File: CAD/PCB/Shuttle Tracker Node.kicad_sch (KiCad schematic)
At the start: 23 parts, among them J1 Conn_01x01, J2 Conn_01x01, J3 Conn_01x01, J4 Conn_01x01, J5 Conn_01x01, J6 Conn_01x01, J7 Conn_01x01, SW1 SW_Push, SW10 SW_Push, SW11 SW_Push, SW12 SW_Push, SW13 PEC11-4215F-S24, SW2 SW_Push, SW3 SW_Push, SW4 SW_Push, SW5 SW_Push, SW6 SW_Push, SW7 SW_Push, SW8 SW_Push, SW9 SW_Push, U1 ESP32-C3-DEVKITC-02

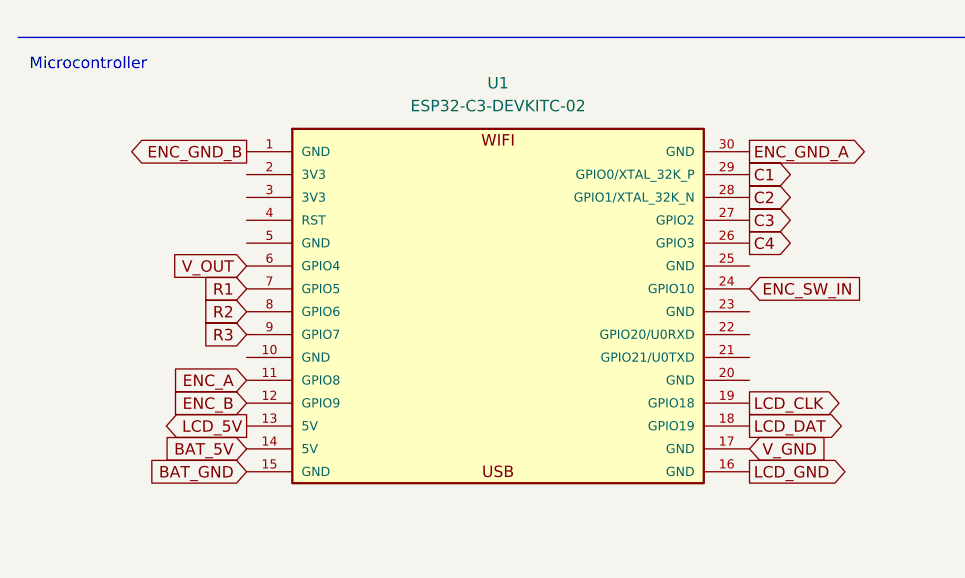
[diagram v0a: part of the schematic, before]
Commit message: Finished PCB Routing
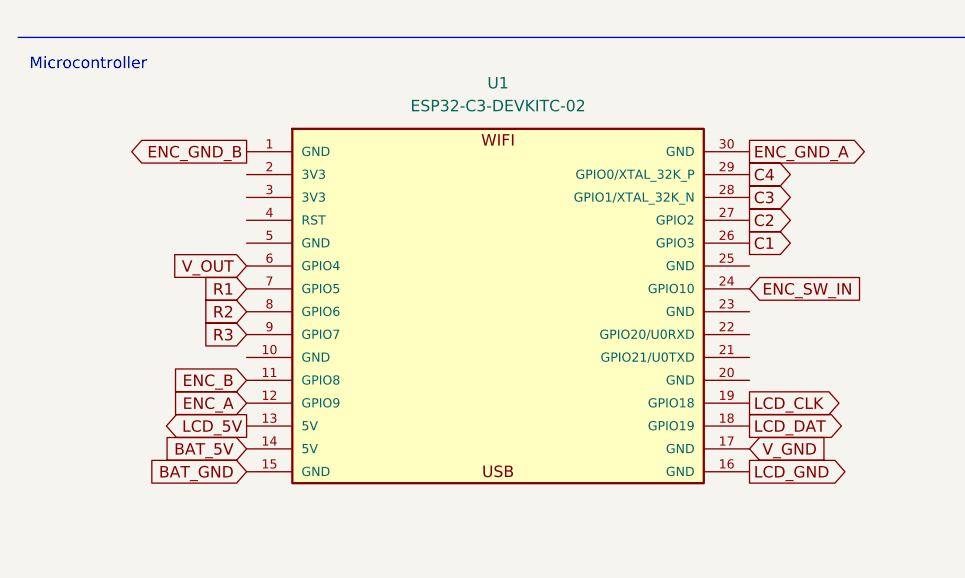
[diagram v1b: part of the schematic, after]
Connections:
- net C1: now also U1.26 (GPIO3); no longer U1.29 (GPIO0/XTAL_32K_P)
- net C2: now also U1.27 (GPIO2); no longer U1.28 (GPIO1/XTAL_32K_N)
- net C3: now also U1.28 (GPIO1/XTAL_32K_N); no longer U1.27 (GPIO2)
- net C4: now also U1.29 (GPIO0/XTAL_32K_P); no longer U1.26 (GPIO3)
- net ENC_A: now also U1.12 (GPIO9); no longer U1.11 (GPIO8)
- net ENC_B: now also U1.11 (GPIO8); no longer U1.12 (GPIO9)
